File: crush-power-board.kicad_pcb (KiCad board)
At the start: 4 copper layers, 138.8 x 128.2 mm, 105 parts, among them J1 XT90PW-F, J2 1x2 Header, J3 Molex Micro Fit 3.0, J4 Barrel_Jack, J5 2157601008, U1 BD9G341AEFJ, U2 SIC461ED-T1-GE3, U3 SIC461ED-T1-GE3, U4 BD9G341AEFJ

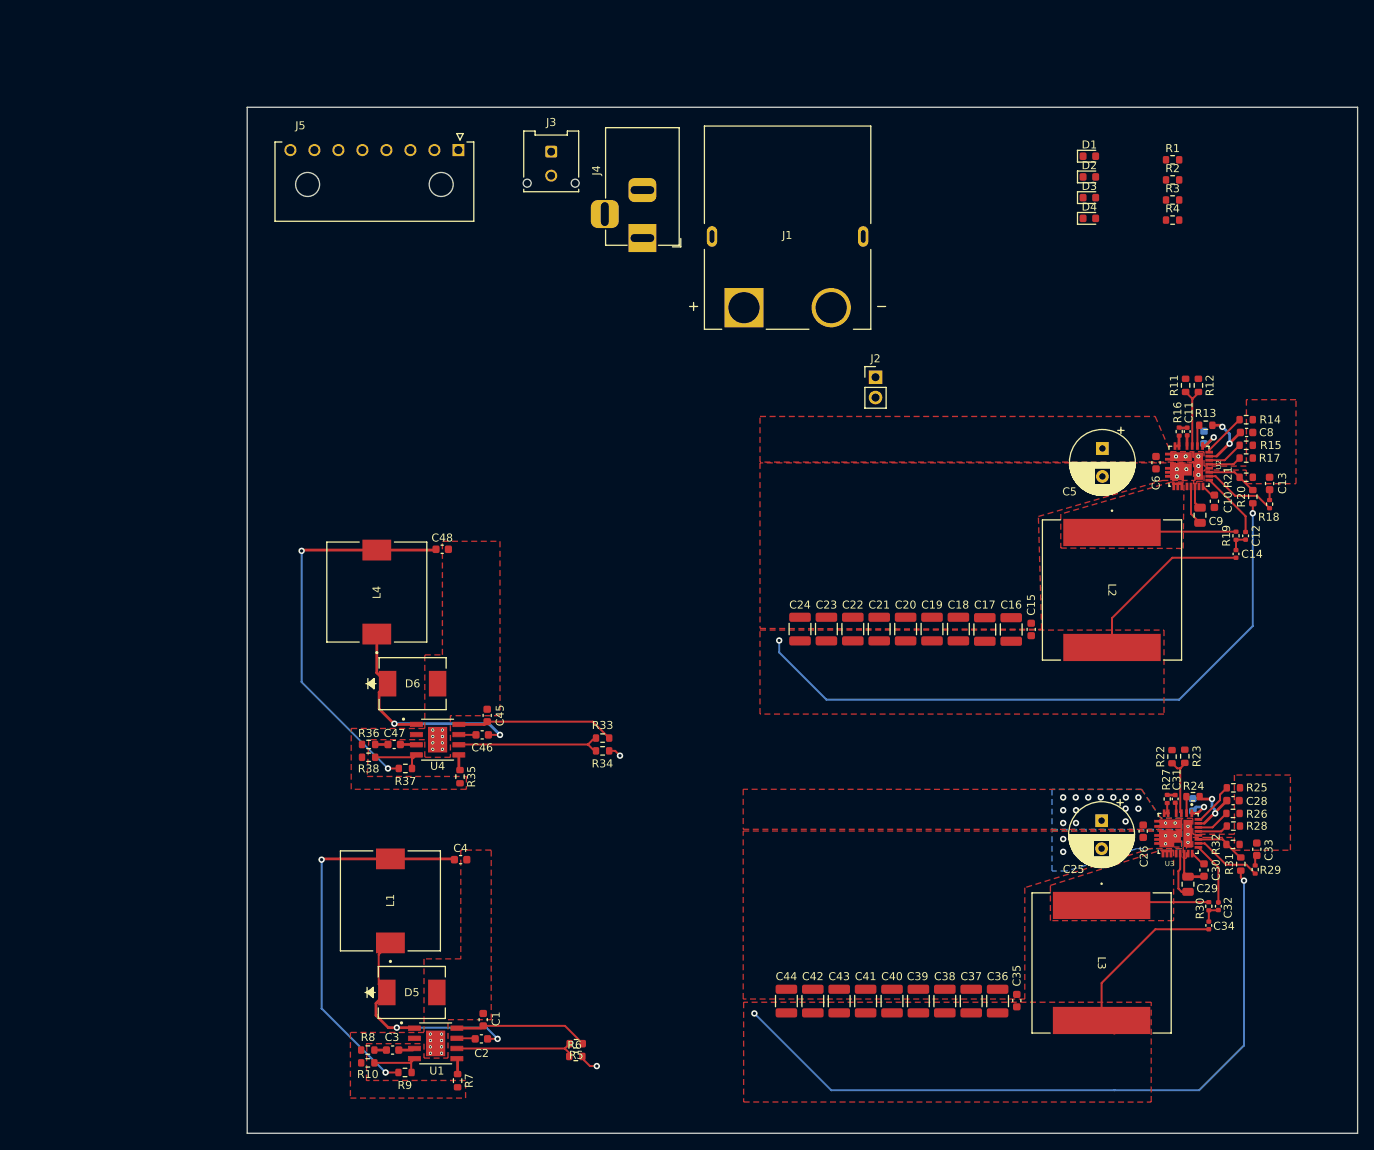
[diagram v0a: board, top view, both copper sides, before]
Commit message: preparing for board layout
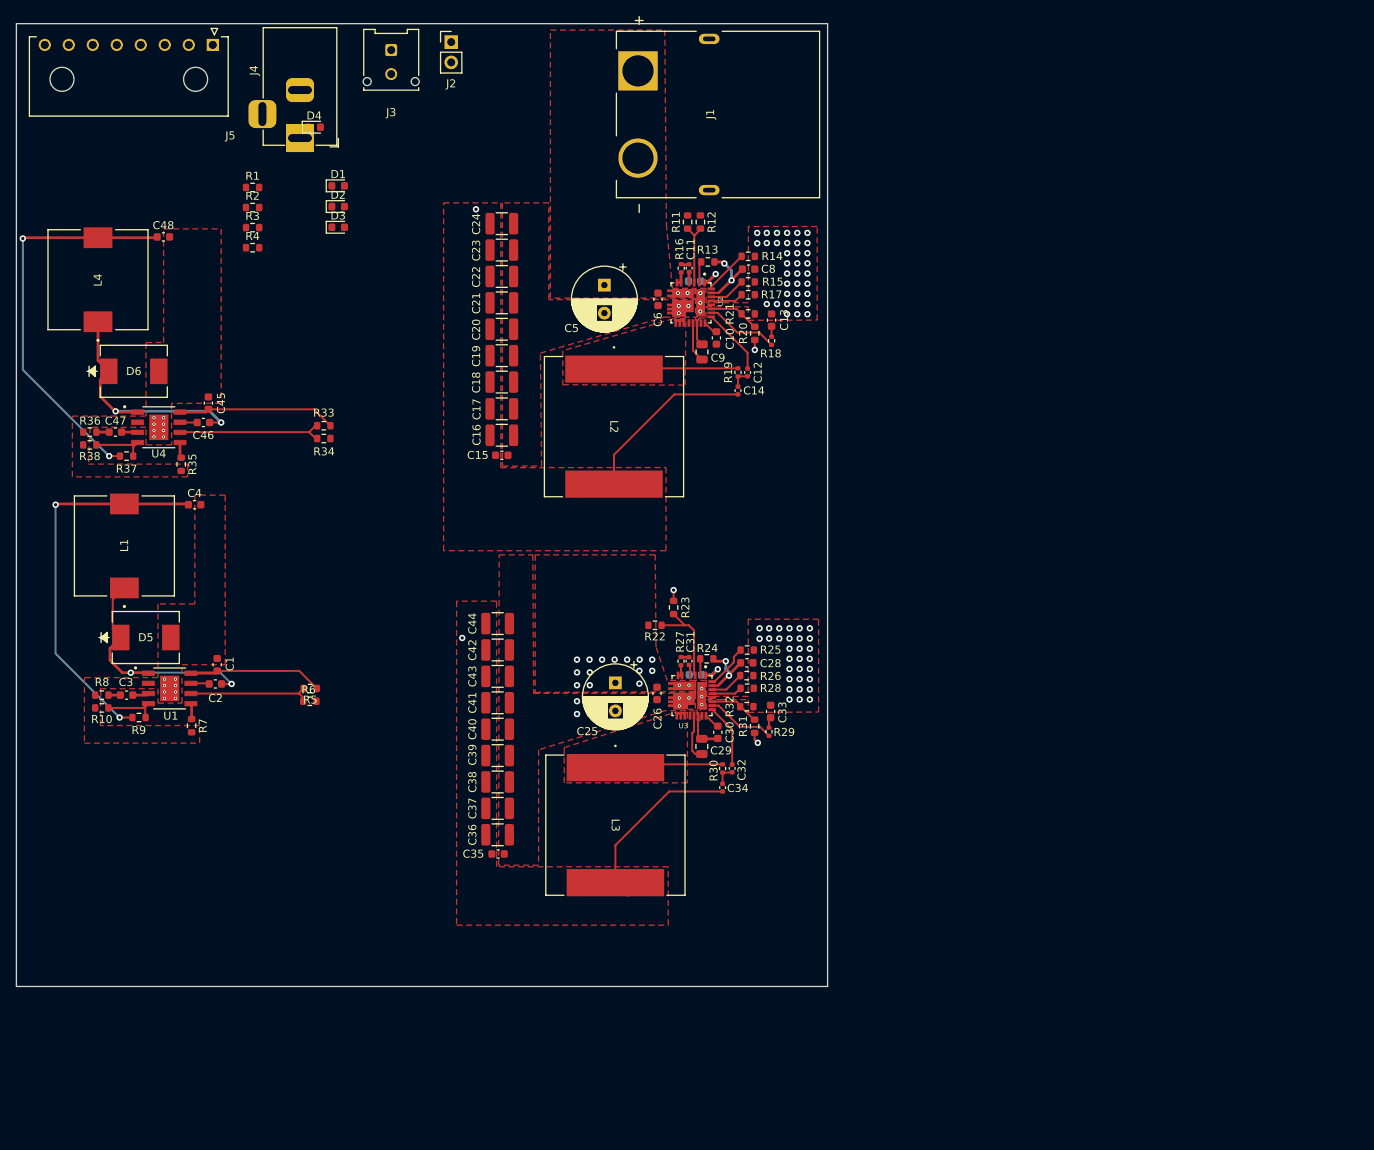
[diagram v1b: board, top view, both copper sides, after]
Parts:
- moved R1 115.1 mm to (42.4, 33.4)
- moved R2 115.1 mm to (42.4, 35.9)
- moved R3 115.1 mm to (42.4, 38.4)
- moved R4 115.1 mm to (42.4, 40.9)
- moved D4 97.6 mm to (50.1, 25.8)
- moved D1 94.0 mm to (53.1, 33.2)
- moved D2 94.0 mm to (53.1, 35.8)
- moved D3 94.0 mm to (53.1, 38.4)
- moved C15 69.7 mm to (73.5, 66.8), turned to 0 degrees
- moved C16 68.1 mm to (73.5, 64.3), turned to 0 degrees
- moved J2 67.6 mm to (67.2, 15.2)
- moved C35 67.4 mm to (73.1, 116.7), turned to 0 degrees
- moved R22 66.7 mm to (92.7, 88.1), turned to 180 degrees
- moved C7 66.6 mm to (97.6, 45.1), turned to 0 degrees
- moved R23 66.6 mm to (95.0, 85.9)
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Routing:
- net 12V: track 104.6 -> 118.4 mm
- net 5V: track 112.9 -> 121.2 mm
- net Net-(U3-EN): track 7.77 -> 12.0 mm
- net GND1: track 1.60 -> 0.00 mm, vias 9 -> 8
- net +BATT: track 24.0 -> 25.3 mm
- net GND: track 10.7 -> 9.65 mm, vias 27 -> 92
- added copper zone on In2.Cu, net GND
- removed copper zone on B.Cu, net +BATT
- removed copper zone on B.Cu, net GND
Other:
- board size 138.8 x 128.2 mm -> 101.4 x 120.3 mm
